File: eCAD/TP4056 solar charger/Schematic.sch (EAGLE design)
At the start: 19 parts, among them IC1 TP4056X, IC2 AP9101CK6-ADTRG1, IC3 FDS6898A, Q1 SI2347DS-T1-GE3

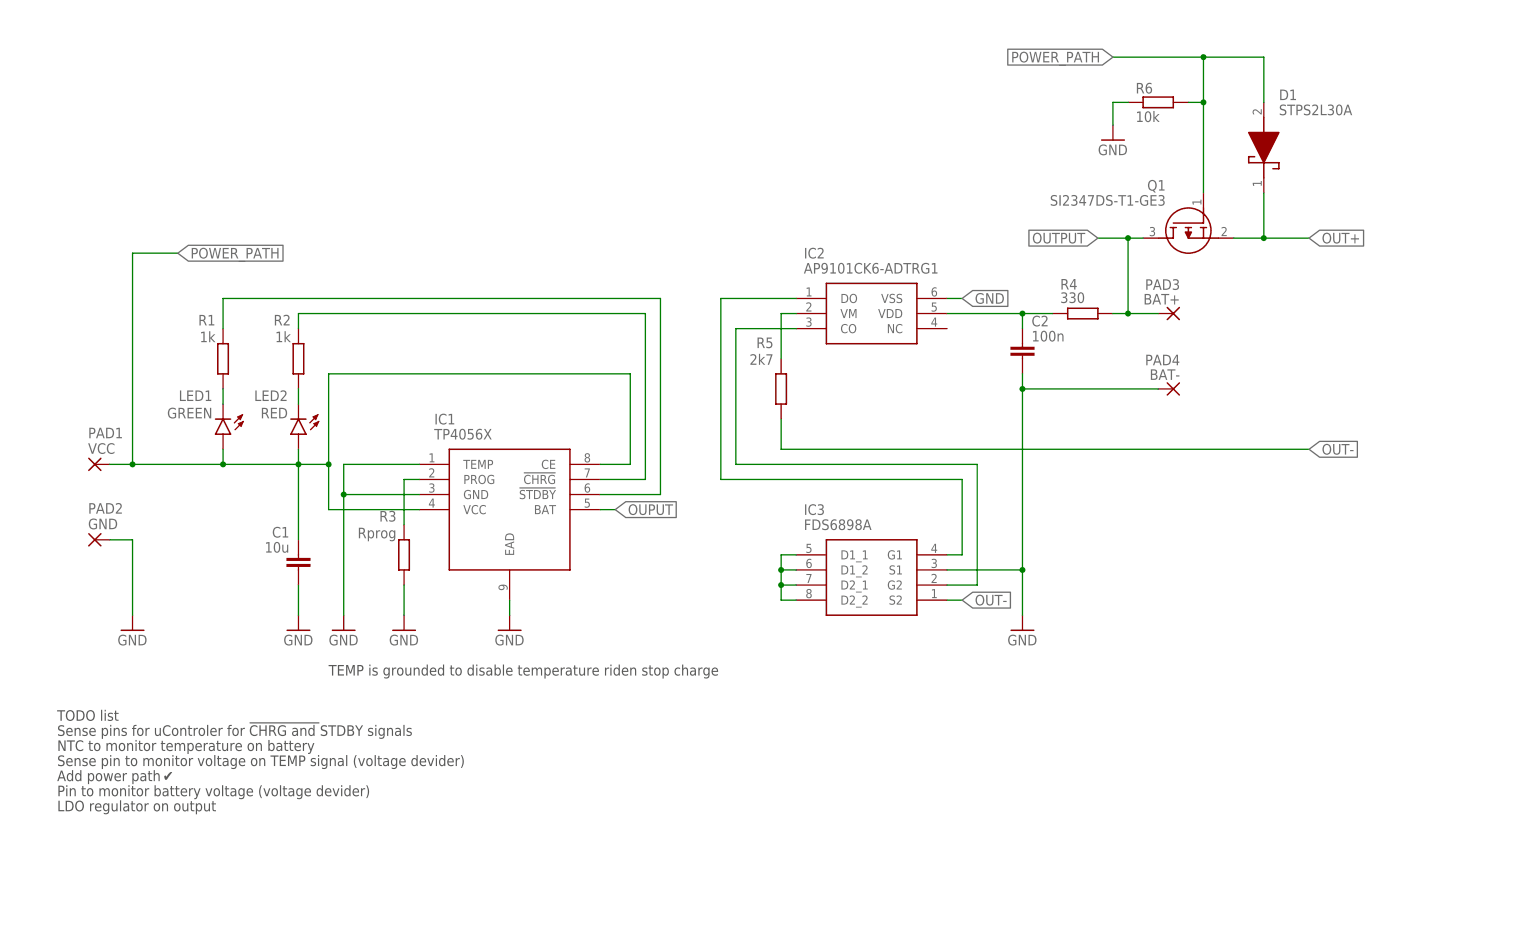
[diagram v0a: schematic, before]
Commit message: Board design
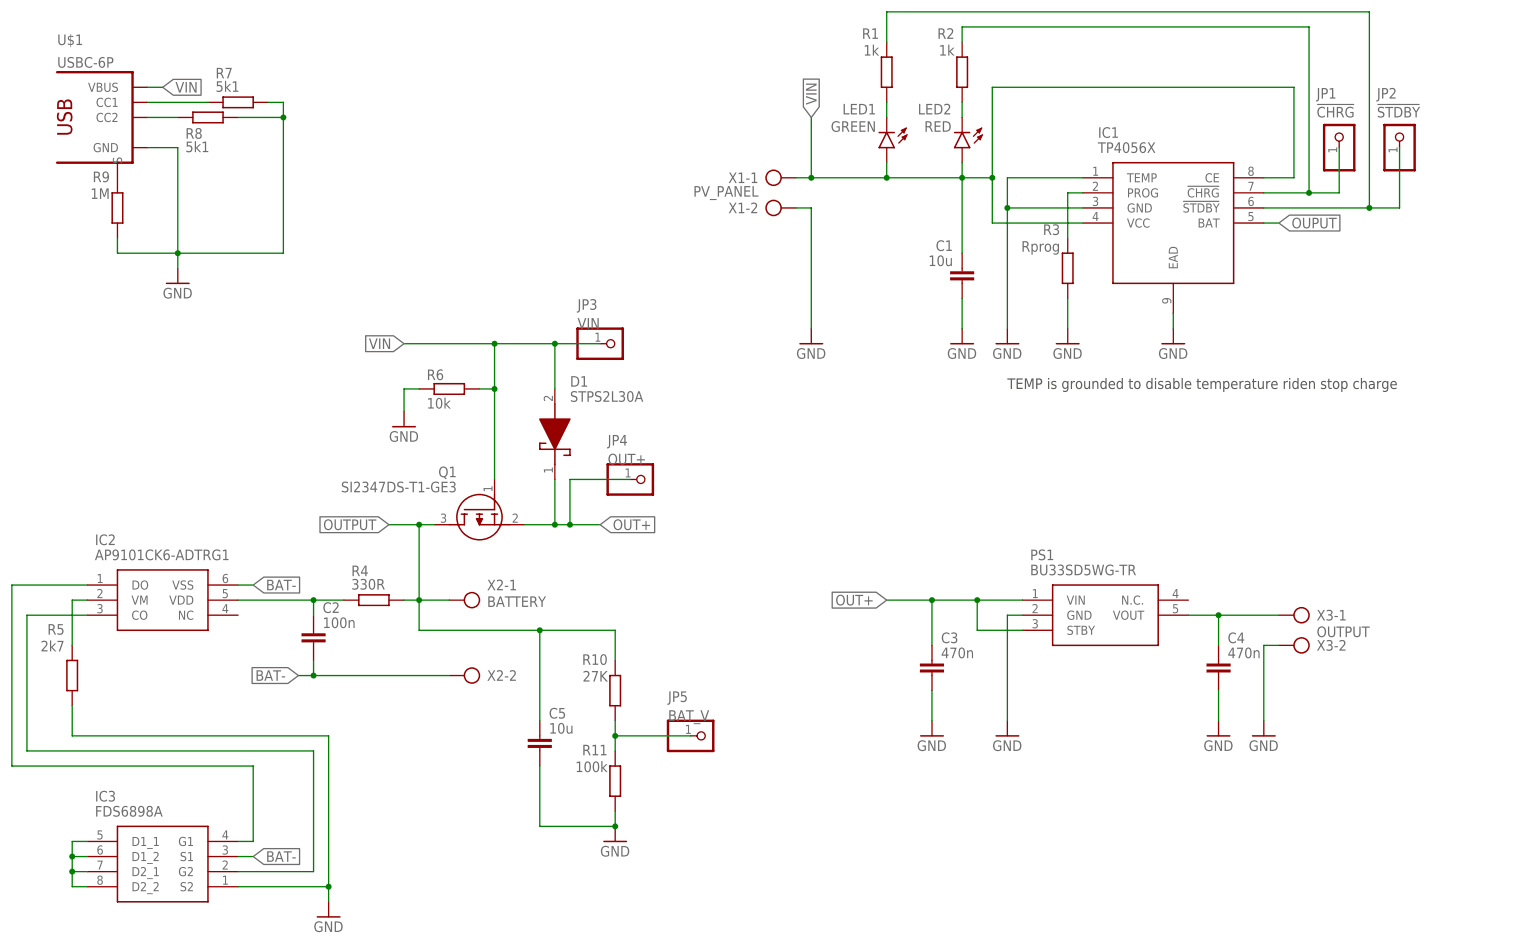
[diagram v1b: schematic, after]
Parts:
- removed PAD1: VCC, wirepad:1,6/0,8
- removed PAD2: GND, wirepad:1,6/0,8
- removed PAD3: BAT+, wirepad:1,6/0,8
- removed PAD4: BAT-, wirepad:1,6/0,8
- added C3, C4: 470n, rcl:C-EUC0805
- added C5: 10u, rcl:C-EUC0805
- added JP1: !CHRG, pinhead:PINHD-1X1
- added JP2: !STDBY, pinhead:PINHD-1X1
- added JP3: VIN, pinhead:PINHD-1X1
- added JP4: OUT+, pinhead:PINHD-1X1
- added JP5: BAT_V, pinhead:PINHD-1X1
- added PS1: BU33SD5WG-TR, 1-component-search:BU33SD5WG-TR
- added R10: 27K, rcl:R-EU_R0805
- added R11: 100k, rcl:R-EU_R0805
- added R7, R8: 5k1, rcl:R-EU_R0805
- added R9: 1M, rcl:R-EU_R0805
- added U$1: USBC-6P, USBC6P:USBC-6P
- added X1: PV_PANEL, con-ptr500:AK300/2
- added X2: BATTERY, con-ptr500:AK300/2
- added X3: OUTPUT, con-ptr500:AK300/2
- R4: value 330 -> 330R
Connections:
- removed net OUT-: IC3.S2, R5.1
- removed net POWER_PATH: C1.1, D1.A, IC1.CE, IC1.VCC, LED1.A, LED2.A, PAD1.P, Q1.G, R6.2
- new net BAT-: C2.2, IC2.VSS, IC3.S1, X2-2.KL
- new net N$11: R7.2, U$1.CC1
- new net N$14: C4.1, PS1.VOUT, X3-1.KL
- new net N$15: JP5.1, R10.1, R11.2
- new net N$7: R9.1, U$1.S
- new net N$8: R8.2, U$1.CC2
- new net VIN: C1.1, D1.A, IC1.CE, IC1.VCC, JP3.1, LED1.A, LED2.A, Q1.G, R6.2, U$1.VBUS, X1-1.KL
- net GND: now also C3.2, C4.2, C5.2, IC3.S2, PS1.GND, R11.1, R5.1, R7.1, R8.1, R9.2, U$1.GND, X1-2.KL, X3-2.KL; no longer C2.2, IC2.VSS, IC3.S1, PAD2.P, PAD4.P
- net N$3: now also JP2.1
- net N$6: now also JP1.1
- net OUT+: now also C3.1, JP4.1, PS1.STBY, PS1.VIN
- net OUTPUT: now also C5.1, R10.2, X2-1.KL; no longer PAD3.P
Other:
- note removed: "Add power path"
- note removed: "LDO regulator on output"
- note removed: "NTC to monitor temperature on battery"
- note removed: "Pin to monitor battery voltage (voltage devider)"
- note removed: "Sense pin to monitor voltage on TEMP signal (voltage devider)"
- note removed: "Sense pins for uControler for !CHRG and !STDBY signals"
- note removed: "TODO list"
- note removed: "✔"
- moved on the sheet: C1, C2, D1, IC1, IC2, IC3, LED1, LED2, Q1, R1, R2, R3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
